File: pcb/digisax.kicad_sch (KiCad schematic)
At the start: 27 parts, among them U1 TLV320DAC3100_breakout, U2 MPXV7007, U3 ESP32-S3, U4 MCP3221

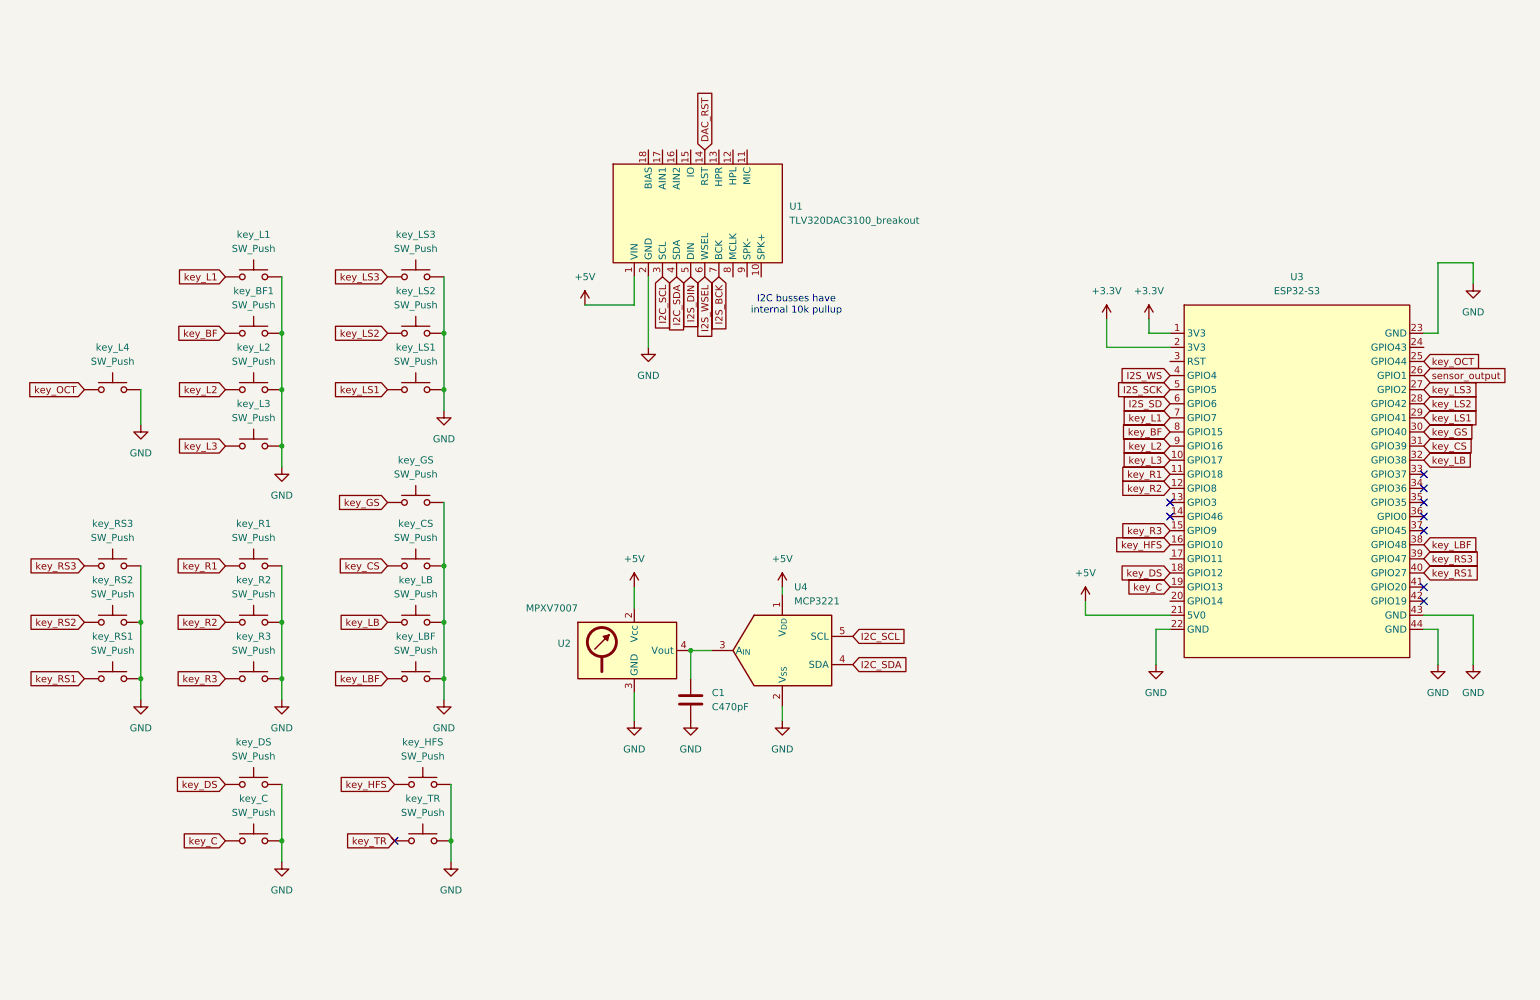
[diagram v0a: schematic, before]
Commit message: started matrix wiring
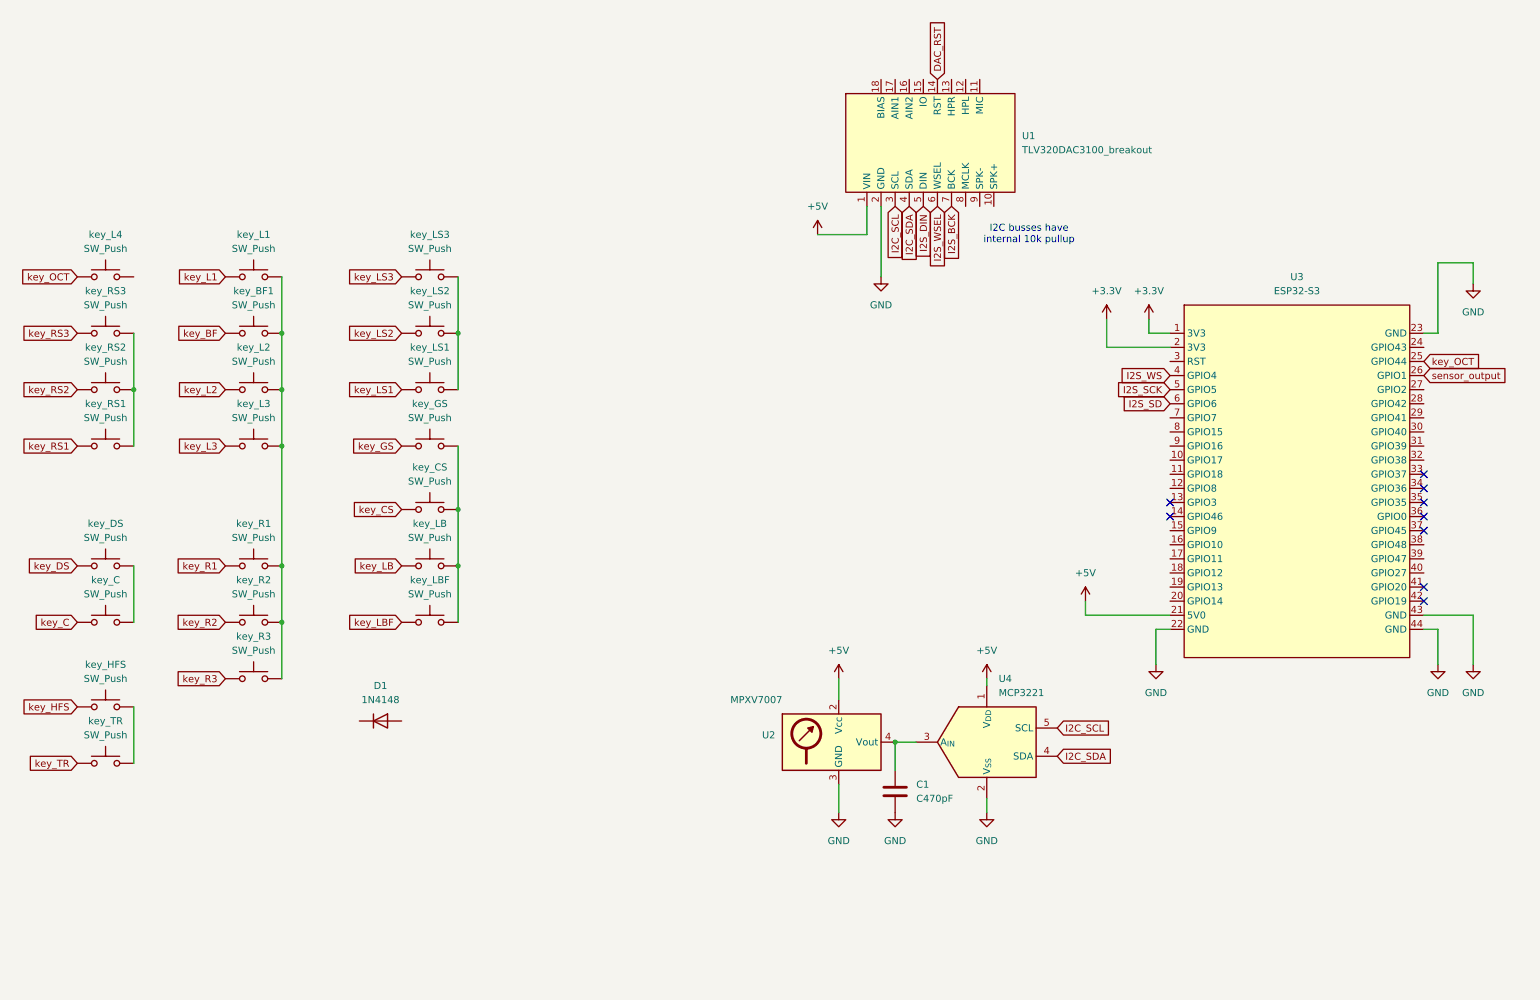
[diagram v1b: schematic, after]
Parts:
- added D1: 1N4148, Diode_THT:D_DO-35_SOD27_P7.62mm_Horizontal, symbol Diode:1N4148
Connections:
- net GND: no longer key_BF1.2, key_C.2, key_CS.2, key_DS.2, key_GS.2, key_HFS.2, key_L1.2, key_L2.2, key_L3.2, key_L4.2, key_LB.2, key_LBF.2, key_LS1.2, key_LS2.2, key_LS3.2, key_R1.2, key_R2.2, key_R3.2, key_RS1.2, key_RS2.2, key_RS3.2, key_TR.2
- net key_BF: no longer U3.8 (GPIO15)
- net key_C: no longer U3.19 (GPIO13)
- net key_CS: no longer U3.31 (GPIO39)
- net key_DS: no longer U3.18 (GPIO12)
- net key_GS: no longer U3.30 (GPIO40)
- net key_HFS: no longer U3.16 (GPIO10)
- net key_L1: no longer U3.7 (GPIO7)
- net key_L2: no longer U3.9 (GPIO16)
- net key_L3: no longer U3.10 (GPIO17)
- net key_LB: no longer U3.32 (GPIO38)
- net key_LBF: no longer U3.38 (GPIO48)
- net key_LS1: no longer U3.29 (GPIO41)
- net key_LS2: no longer U3.28 (GPIO42)
- net key_LS3: no longer U3.27 (GPIO2)
- net key_R1: no longer U3.11 (GPIO18)
- net key_R2: no longer U3.12 (GPIO8)
- net key_R3: no longer U3.15 (GPIO9)
- net key_RS1: no longer U3.40 (GPIO27)
- net key_RS3: no longer U3.39 (GPIO47)
- new net: key_BF1.2, key_L1.2, key_L2.2, key_L3.2, key_R1.2, key_R2.2, key_R3.2
- new net: key_LS1.2, key_LS2.2, key_LS3.2
- new net: key_C.2, key_DS.2
- new net: key_CS.2, key_GS.2, key_LB.2, key_LBF.2
- new net: key_RS1.2, key_RS2.2, key_RS3.2
- new net: key_HFS.2, key_TR.2
- no-connect marks 10 -> 9
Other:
- moved on the sheet: C1, U1, U2, U4, key_C, key_CS, key_DS, key_GS, key_HFS, key_L4, key_LB, key_LBF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

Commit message: completed first iteration of schem
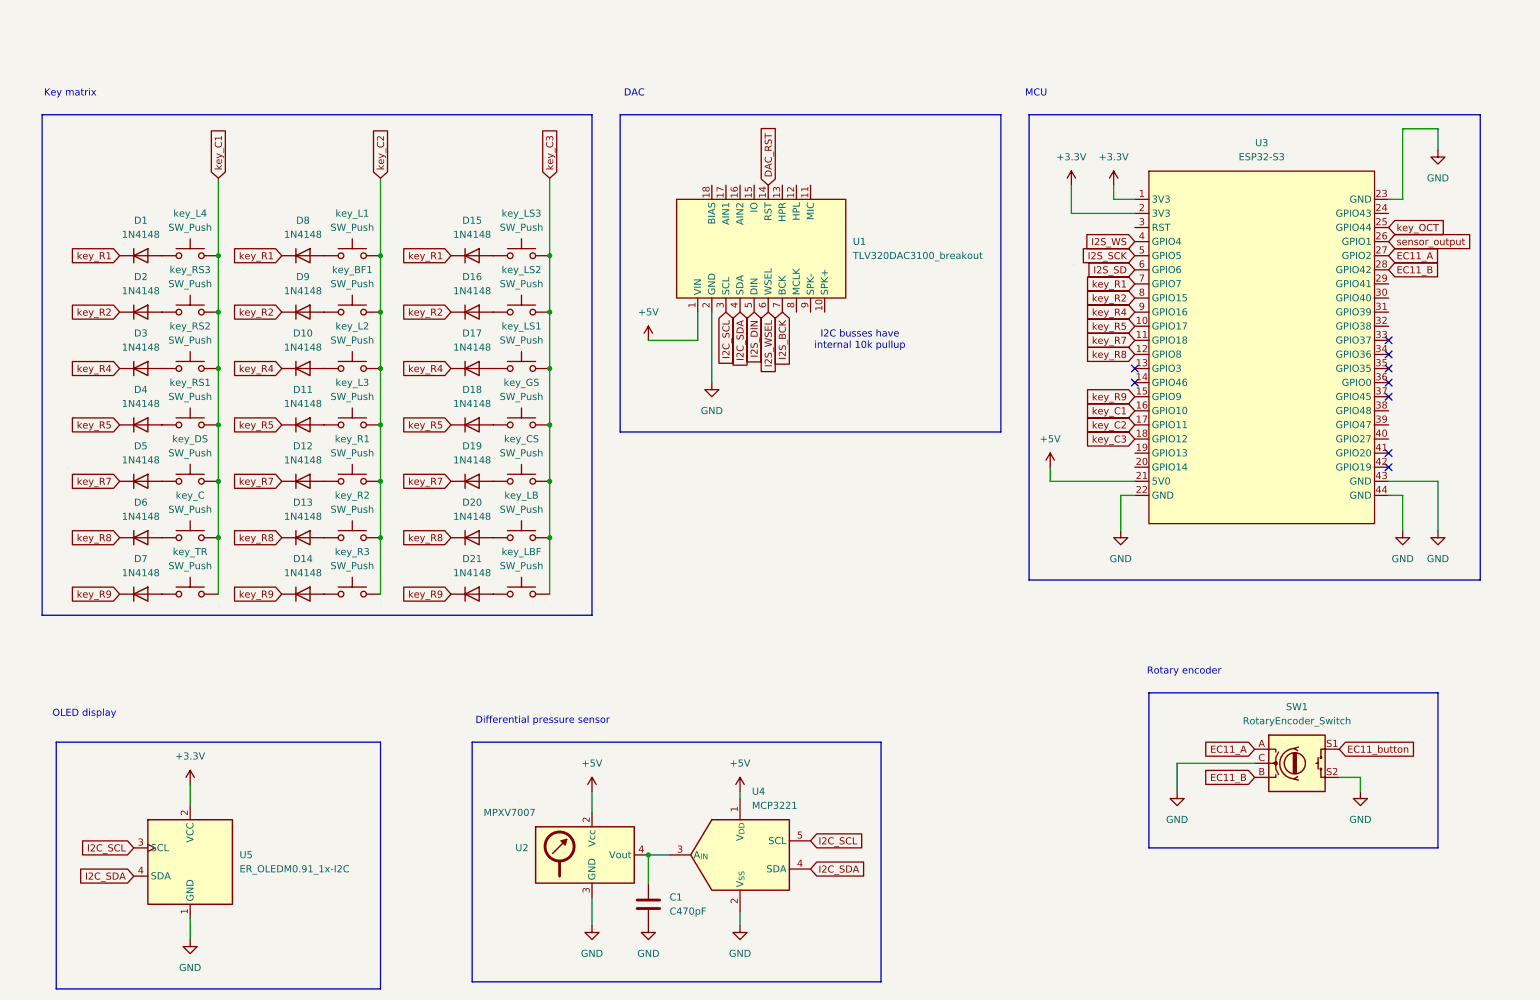
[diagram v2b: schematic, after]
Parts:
- removed key_HFS: SW_Push, symbol Switch:SW_Push
- added D10, D11, D12, D13, D14, D15, D16, D17, D18, D19, D2, D20, D21, D3, D4, D5, D6, D7, D8, D9: 1N4148, Diode_THT:D_DO-35_SOD27_P7.62mm_Horizontal, symbol Diode:1N4148
- added SW1: RotaryEncoder_Switch, symbol Device:RotaryEncoder_Switch
- added U5: ER_OLEDM0.91_1x-I2C, Display:ER_OLEDM0.91_1x-I2C, symbol Display_Graphic:ER_OLEDM0.91_1x-I2C
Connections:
- net +3.3V: now also U5.2 (VCC)
- net GND: now also SW1.C, SW1.S2, U5.1 (GND)
- net I2C_SCL: now also U5.3 (SCL)
- net I2C_SDA: now also U5.4 (SDA)
- net key_OCT: no longer key_L4.1
- net key_R1: now also D1.1 (K), U3.7 (GPIO7), D15.1 (K), D8.1 (K); no longer key_R1.1
- net key_R2: now also U3.8 (GPIO15), D16.1 (K), D2.1 (K), D9.1 (K); no longer key_R2.1
- net key_C2: now reaches key_BF1.2, key_L1.2, key_L2.2, key_L3.2, key_R1.2, key_R2.2, key_R3.2
- net key_C2: now also U3.17 (GPIO11)
- net key_C3: now reaches key_LS1.2, key_LS2.2, key_LS3.2
- net key_C3: now also U3.18 (GPIO12), key_CS.2, key_GS.2, key_LB.2, key_LBF.2
- net key_C1: now reaches key_C.2, key_DS.2
- net key_C1: now also U3.16 (GPIO10), key_L4.2, key_RS1.2, key_RS2.2, key_RS3.2, key_TR.2
- net key_R5: now reaches U3.10 (GPIO17)
- net key_R5: now also D11.1 (K), D18.1 (K), D4.1 (K)
- net key_R7: now reaches U3.11 (GPIO18)
- net key_R7: now also D12.1 (K), D19.1 (K), D5.1 (K)
- net key_R8: now reaches U3.12 (GPIO8)
- net key_R8: now also D13.1 (K), D20.1 (K), D6.1 (K)
- net key_R9: now reaches U3.15 (GPIO9)
- net key_R9: now also D14.1 (K), D21.1 (K), D7.1 (K)
- net EC11_A: now reaches U3.27 (GPIO2)
- net EC11_A: now also SW1.A
- net EC11_B: now reaches U3.28 (GPIO42)
- net EC11_B: now also SW1.B
- net key_R4: now reaches U3.9 (GPIO16)
- net key_R4: now also D10.1 (K), D17.1 (K), D3.1 (K)
- net at D1.2 (A): now also key_L4.1
- net key_BF: no longer names the net of key_BF1.1
- net key_BF: now also D9.2 (A)
- net key_C: no longer names the net of key_C.1
- net key_C: now also D6.2 (A)
- net key_CS: no longer names the net of key_CS.1
- net key_CS: now also D19.2 (A)
- net key_DS: no longer names the net of key_DS.1
- net key_DS: now also D5.2 (A)
- net key_GS: no longer names the net of key_GS.1
- net key_GS: now also D18.2 (A)
- net key_L1: no longer names the net of key_L1.1
- net key_L1: now also D8.2 (A)
- net key_L2: no longer names the net of key_L2.1
- net key_L2: now also D10.2 (A)
- net key_L3: no longer names the net of key_L3.1
- net key_L3: now also D11.2 (A)
- net key_LB: no longer names the net of key_LB.1
- net key_LB: now also D20.2 (A)
- net key_LBF: no longer names the net of key_LBF.1
- net key_LBF: now also D21.2 (A)
- net key_LS1: no longer names the net of key_LS1.1
- net key_LS1: now also D17.2 (A)
- net key_LS2: no longer names the net of key_LS2.1
- net key_LS2: now also D16.2 (A)
- net key_LS3: no longer names the net of key_LS3.1
- net key_LS3: now also D15.2 (A)
- net key_R3: no longer names the net of key_R3.1
- net key_R3: now also D14.2 (A)
- net key_RS1: no longer names the net of key_RS1.1
- net key_RS1: now also D4.2 (A)
- net key_RS2: no longer names the net of key_RS2.1
- net key_RS2: now also D3.2 (A)
- net key_RS3: no longer names the net of key_RS3.1
- net key_RS3: now also D2.2 (A)
- net key_TR: no longer names the net of key_TR.1
- net key_TR: now also D7.2 (A)
- new net: D13.2 (A), key_R2.1
- new net: D12.2 (A), key_R1.1
- new net EC11_button: SW1.S1
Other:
- note added: "DAC"
- note added: "Differential pressure sensor"
- note added: "Key matrix"
- note added: "MCU"
- note added: "OLED display"
- note added: "Rotary encoder"
- moved on the sheet: C1, D1, U1, U2, U3, U4, key_BF1, key_C, key_CS, key_DS, key_GS, key_L1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
